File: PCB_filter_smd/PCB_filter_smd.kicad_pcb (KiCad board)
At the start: 2 copper layers, 25 parts, among them J1 Conn_01x02_Pin, J2 Conn_01x02_Pin, U1 AD620, U2 LM324

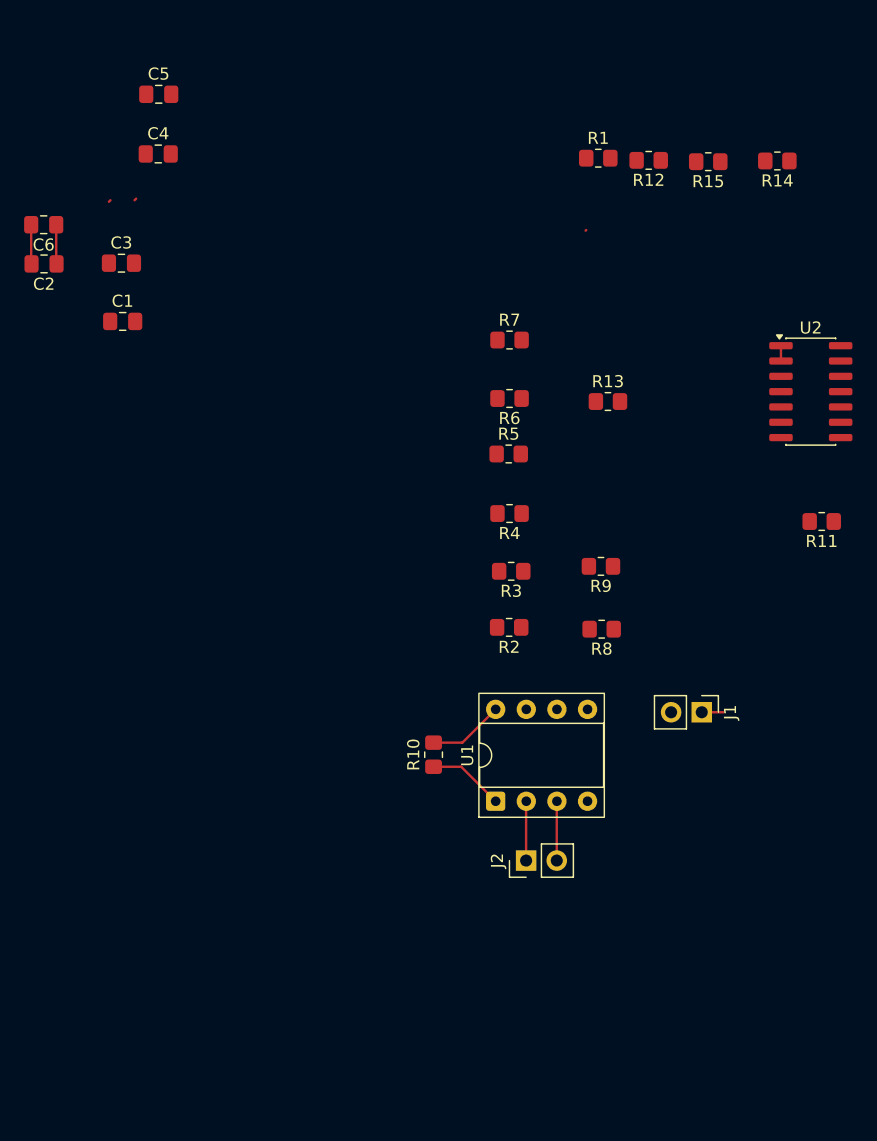
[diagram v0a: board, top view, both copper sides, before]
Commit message: last
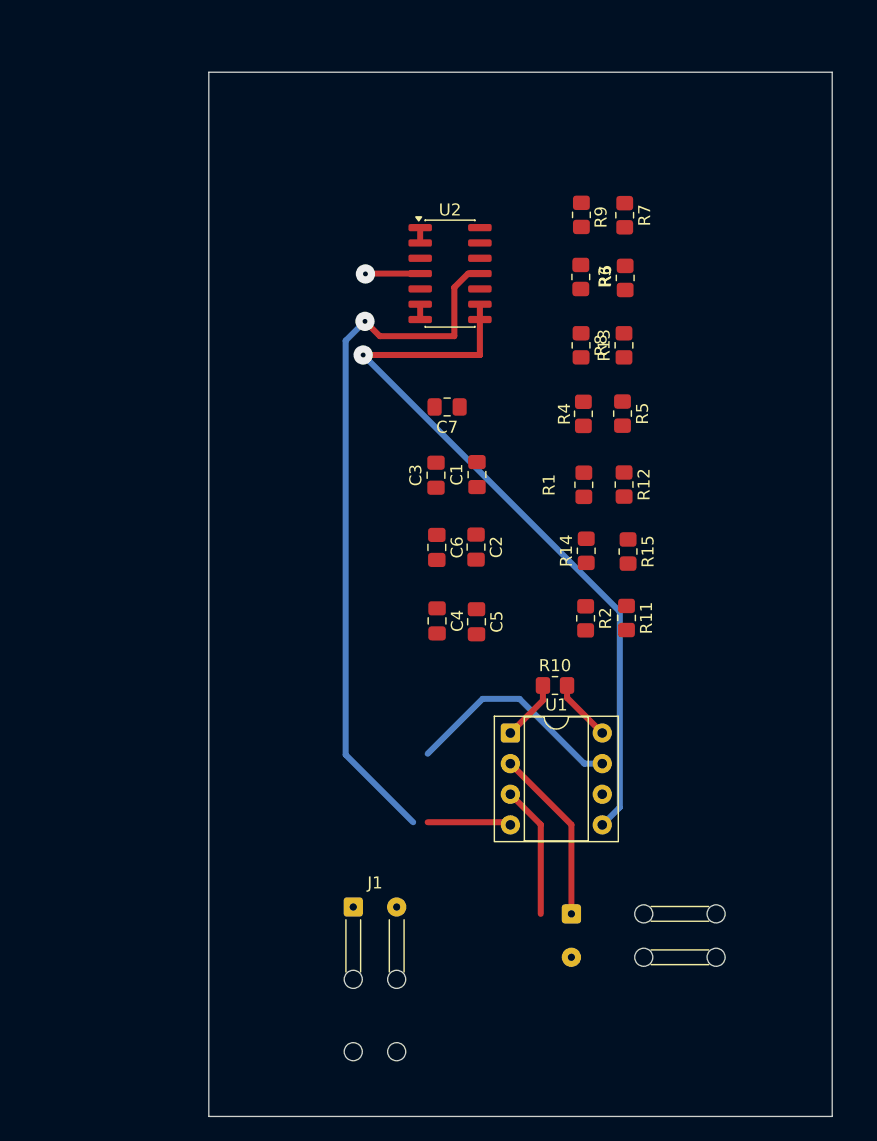
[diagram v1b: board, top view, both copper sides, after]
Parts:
- added C7: 10n, Capacitor_SMD:C_0805_2012Metric_Pad1.18x1.45mm_HandSolder, F.Cu at (120.8, 87.3)
- J1: footprint Connector_PinHeader_2.54mm:PinHeader_1x02_P2.54mm_Vertical -> Connector_Wire:SolderWire-0.1sqmm_1x02_P3.6mm_D0.4mm_OD1mm_Relief2x
- J2: footprint Connector_PinHeader_2.54mm:PinHeader_1x02_P2.54mm_Vertical -> Connector_Wire:SolderWire-0.1sqmm_1x02_P3.6mm_D0.4mm_OD1mm_Relief2x; moved to B.Cu
- moved C5 51.1 mm to (123.3, 105.1), turned to -90 degrees
- moved C4 45.1 mm to (120.0, 105.1), turned to -90 degrees
- moved C2 42.8 mm to (123.2, 99.0), turned to -90 degrees
- moved C6 42.2 mm to (120.0, 99.0), turned to -90 degrees
- moved R14 36.0 mm to (132.4, 99.3), turned to 90 degrees
- moved J1 33.1 mm to (113.0, 128.8), turned to 0 degrees
- moved R15 33.0 mm to (135.8, 99.3), turned to -90 degrees
- moved C1 32.0 mm to (123.3, 92.9), turned to 90 degrees
- moved U2 31.5 mm to (121.1, 76.3)
- moved C3 31.5 mm to (119.9, 93.0), turned to 90 degrees
- moved R9 29.2 mm to (132.0, 71.4), turned to -90 degrees
- moved R1 27.1 mm to (132.2, 93.8), turned to -90 degrees
- moved R12 27.0 mm to (135.5, 93.8), turned to -90 degrees
- moved R3 25.1 mm to (131.9, 76.5), turned to -90 degrees
- moved R8 23.6 mm to (131.9, 82.2), turned to -90 degrees
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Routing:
- net GND: track 1.23 -> 66.0 mm, vias 0 -> 1
- net VGND: track 0.00 -> 62.3 mm, vias 0 -> 1
- net VCC: track 2.61 -> 23.1 mm, vias 0 -> 1
- net Net-(J2-Pin_1): track 4.93 -> 14.6 mm
- net Net-(J2-Pin_2): track 4.93 -> 11.0 mm
- net Net-(C2-Pad2): track 3.42 -> 0.00 mm
- net Net-(U2A--): track 4.53 -> 1.27 mm
- net Net-(R10-Pad1): track 6.33 -> 5.06 mm
- net Net-(U2B--): track 0.08 -> 1.27 mm
- net Net-(R10-Pad2): track 6.29 -> 5.15 mm
- net Net-(U2D--): track 0.50 -> 0.00 mm
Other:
- board outline added: 51.7 x 86.6 mm

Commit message: last
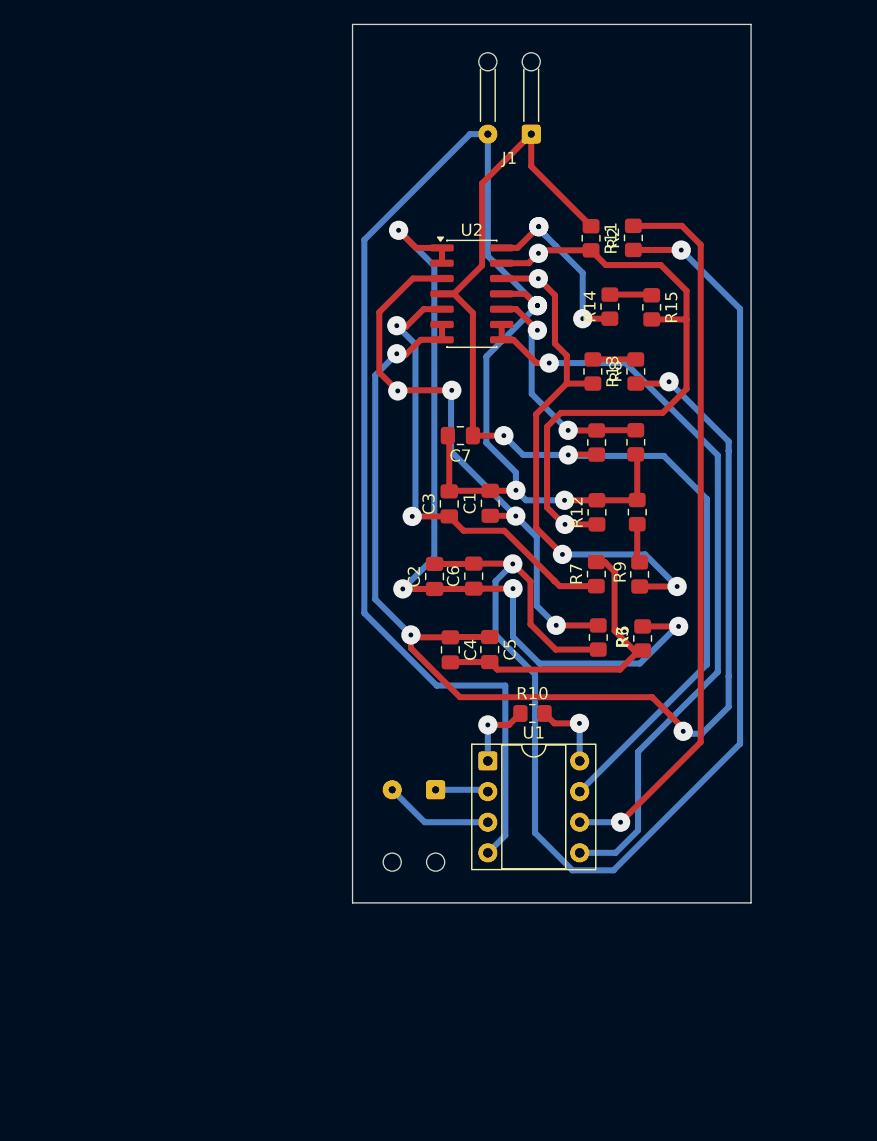
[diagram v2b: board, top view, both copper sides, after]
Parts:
- J1, J2: footprint Connector_Wire:SolderWire-0.1sqmm_1x02_P3.6mm_D0.4mm_OD1mm_Relief2x -> Connector_Wire:SolderWire-0.1sqmm_1x02_P3.6mm_D0.4mm_OD1mm_Relief
- moved J1 65.8 mm to (127.8, 64.7), turned to 180 degrees
- moved R2 31.8 mm to (136.3, 73.3), turned to 90 degrees
- moved R11 31.6 mm to (132.8, 73.3)
- moved R9 30.2 mm to (136.8, 101.2), turned to 90 degrees
- moved R3 29.9 mm to (133.4, 106.5)
- moved R6 29.9 mm to (137.1, 106.5)
- moved R7 29.9 mm to (133.2, 101.2), turned to 90 degrees
- moved R14 20.3 mm to (134.3, 79.0)
- moved R15 20.3 mm to (137.8, 79.1)
- moved J2 15.3 mm to (119.9, 119.1), turned to 180 degrees
- moved R8 5.03 mm to (136.5, 84.4), turned to 90 degrees
- moved R1 4.98 mm to (136.6, 96.0), turned to 90 degrees
- moved C2 4.21 mm to (119.8, 101.4), turned to 90 degrees
- moved C6 3.88 mm to (123.0, 101.4), turned to 90 degrees
- moved R13 3.37 mm to (132.9, 84.4), turned to -90 degrees
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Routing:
- net Net-(C2-Pad2): track 0.00 -> 112.5 mm, vias 0 -> 2
- net Net-(U2B--): track 1.27 -> 100.9 mm, vias 0 -> 4
- net GND: track 66.0 -> 135.6 mm, vias 1 -> 4
- net Net-(U2A--): track 1.27 -> 70.5 mm, vias 0 -> 4
- net VCC: track 23.1 -> 91.6 mm, vias 1 -> 2
- net Net-(R2-Pad2): track 0.00 -> 60.3 mm, vias 0 -> 1
- net Net-(U2D--): track 0.00 -> 52.5 mm, vias 0 -> 2
- net Net-(U2A-+): track 0.00 -> 46.9 mm, vias 0 -> 4
- net Net-(U2D-+): track 0.00 -> 44.9 mm, vias 0 -> 3
- net Net-(U2B-+): track 0.00 -> 39.4 mm, vias 0 -> 2
- net Net-(C4-Pad2): track 0.00 -> 26.6 mm
- net Net-(U2C-+): track 0.00 -> 19.1 mm, vias 0 -> 2
- net Net-(R14-Pad1): track 0.00 -> 15.2 mm, vias 0 -> 3
- net Net-(J2-Pin_1): track 14.6 -> 4.46 mm
- net Net-(R13-Pad1): track 0.00 -> 3.56 mm
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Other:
- board size 51.7 x 86.6 mm -> 33 x 72.9 mm
